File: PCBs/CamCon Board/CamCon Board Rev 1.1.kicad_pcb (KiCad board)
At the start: 2 copper layers, 25 x 25 mm, 28 parts, among them J1 SFW15R-1STE1LF

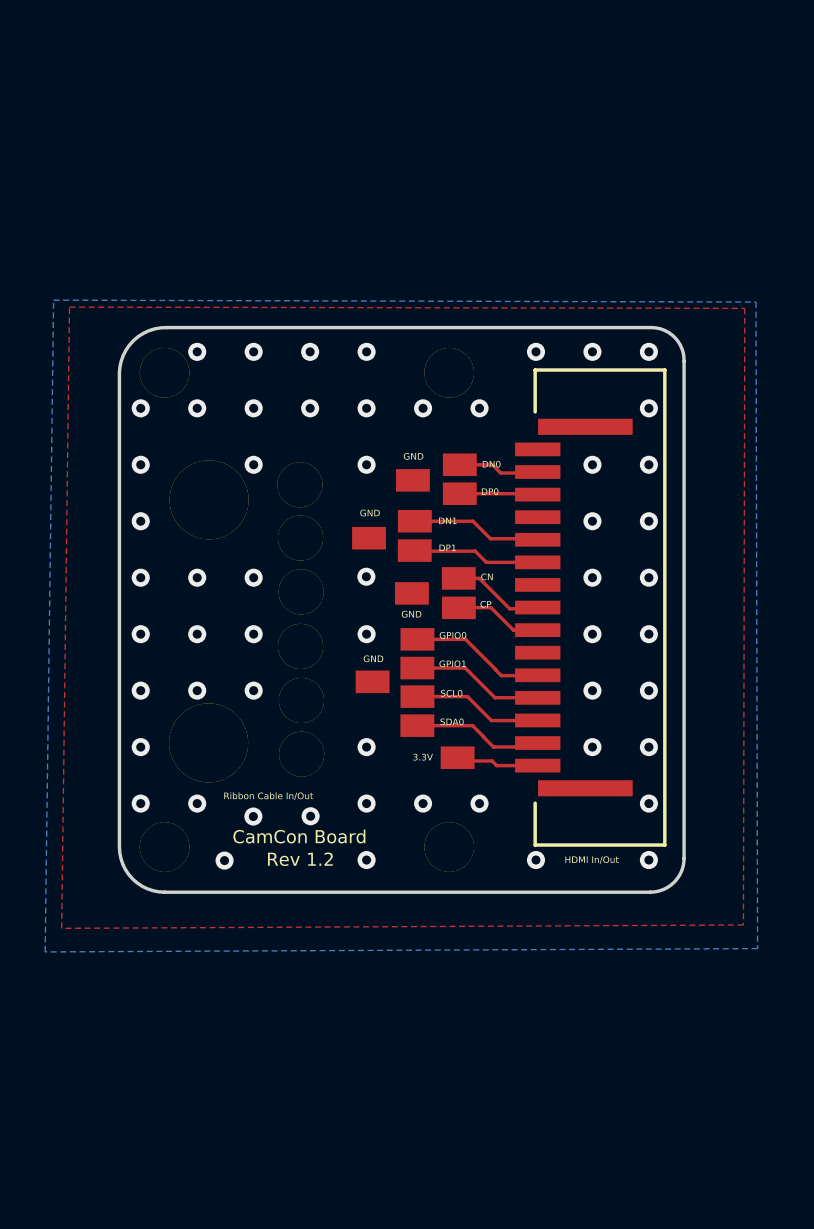
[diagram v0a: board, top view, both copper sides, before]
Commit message: More Gerbers
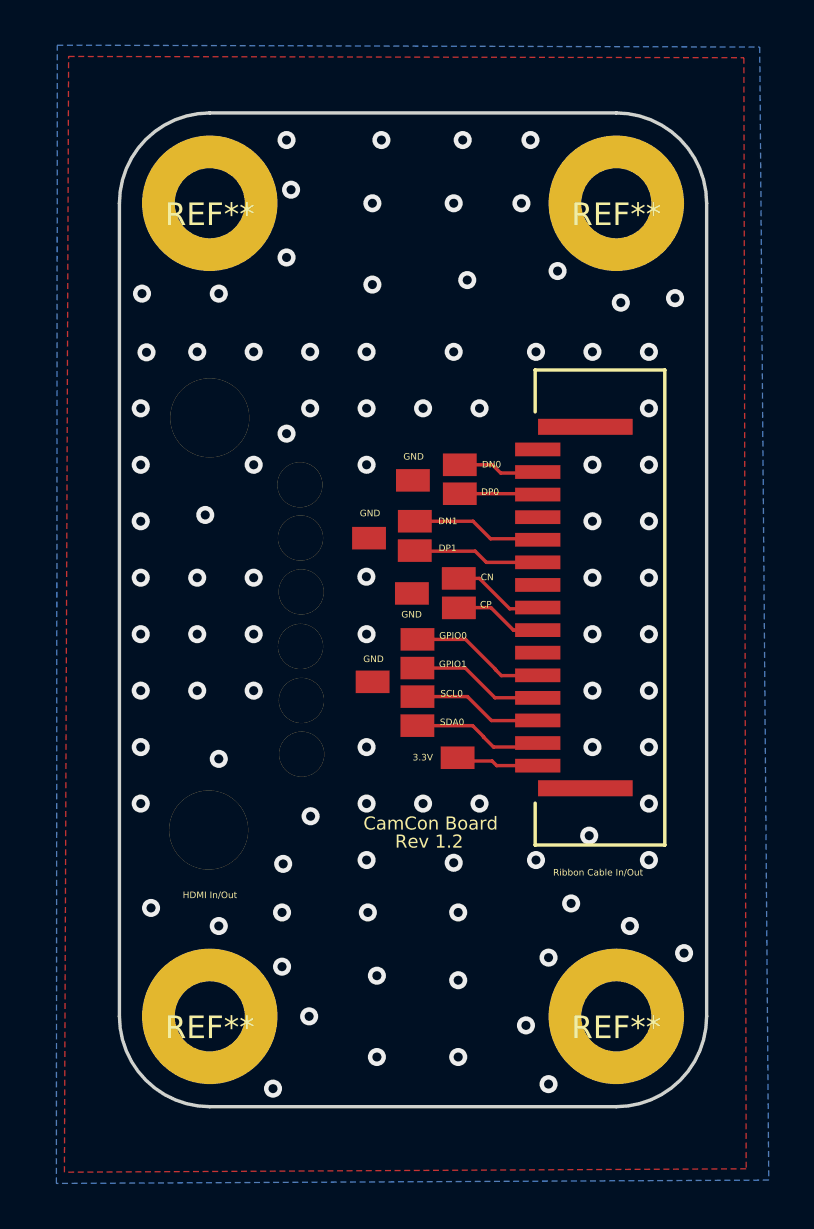
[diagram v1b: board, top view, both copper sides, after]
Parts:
- removed @HOLE0, @HOLE1, @HOLE2, @HOLE3: , 
- added REF**: M3STANDOFF, EER:M3STANDOFF, F.Cu at (140.0, 123.0)
- added REF**: M3STANDOFF, EER:M3STANDOFF, F.Cu at (158.0, 123.0)
- added REF**: M3STANDOFF, EER:M3STANDOFF, F.Cu at (158.0, 87.0)
- added REF**: M3STANDOFF, EER:M3STANDOFF, F.Cu at (140.0, 87.0)
- added U$12: EERLOGO, EER:EERLOGO, B.Cu at (145.8, 114.2)
- moved @HOLE11 3.86 mm to (140.0, 114.8)
- moved @HOLE10 3.63 mm to (140.0, 96.5)
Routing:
- net GND: vias 56 -> 93
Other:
- board size 25 x 25 mm -> 26 x 44 mm

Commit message: 3D Modeling
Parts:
- J1: footprint CamCon Board Rev 1.1:CON15_1X15_DRB_SFW -> EER:CON15_1X15_DRB_SFW
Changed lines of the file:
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@@
     (add_net "Net-(J1-Pad9)")
   )
-  (module EER:M3STANDOFF (layer Top)
-    (at 140 123)
-    (fp_text reference REF** (at 0 0.5) (layer F.SilkS)
-      (effects (font (size 1 1) (thickness 0.15)))
-    )
-    (fp_text value M3STANDOFF (at 0 -0.5) (layer F.Fab)
-      (effects (font (size 1 1) (thickness 0.15)))
-    )
-    (pad 1 thru_hole circle (at 0 0) (size 6 6) (drill 3.1) (layers *.Cu *.Mask))
-  )
-  (module EER:M3STANDOFF (layer Top)
-    (at 158 123)
-    (fp_text reference REF** (at 0 0.5) (layer F.SilkS)
-      (effects (font (size 1 1) (thickness 0.15)))
-    )
-    (fp_text value M3STANDOFF (at 0 -0.5) (layer F.Fab)
-      (effects (font (size 1 1) (thickness 0.15)))
-    )
-    (pad 1 thru_hole circle (at 0 0) (size 6 6) (drill 3.1) (layers *.Cu *.Mask))
-  )
-  (module EER:M3STANDOFF (layer Top)
-    (at 158 87)
-    (fp_text reference REF** (at 0 0.5) (layer F.SilkS)
-      (effects (font (size 1 1) (thickness 0.15)))
-    )
-    (fp_text value M3STANDOFF (at 0 -0.5) (layer F.Fab)
-      (effects (font (size 1 1) (thickness 0.15)))
-    )
-    (pad 1 thru_hole circle (at 0 0) (size 6 6) (drill 3.1) (layers *.Cu *.Mask))
-  )
-  (module "CamCon Board Rev 1.1:CON15_1X15_DRB_SFW" (layer Top)
+  (module EER:CON15_1X15_DRB_SFW (layer Top)
     (at 151.765669 104.898905 270)
     (fp_text reference J1 (at 0 0 270) (layer F.SilkS) hide
@@
     (pad 17 smd rect (at 8.001 -4.8641 270) (size 0.7112 4.191) (layers Top F.Paste F.Mask)
       (net 1 GND) (solder_mask_margin 0.1016))
-    (model "${KIPRJMOD}/3D Components/ssfw15r_2_4st_lf.stp"
-      (offset (xyz 0 8.5 0))
+    (model "../EERLibraries/3D Models/ssfw15r_1_3st_lf.STEP"
+      (offset (xyz -17.3 8.5 2.65))
       (scale (xyz 1 1 1))
-      (rotate (xyz -90 0 180))
+      (rotate (xyz 90 0 0))
     )
   )
+  (module EER:M3STANDOFF (layer Top)
+    (at 140 123)
+    (fp_text reference REF** (at 0 0.5) (layer F.SilkS)
+      (effects (font (size 1 1) (thickness 0.15)))
+    )
+    (fp_text value M3STANDOFF (at 0 -0.5) (layer F.Fab)
+      (effects (font (size 1 1) (thickness 0.15)))
+    )
+    (pad 1 thru_hole circle (at 0 0) (size 6 6) (drill 3.1) (layers *.Cu *.Mask))
+  )
+  (module EER:M3STANDOFF (layer Top)
+    (at 158 123)
+    (fp_text reference REF** (at 0 0.5) (layer F.SilkS)
+      (effects (font (size 1 1) (thickness 0.15)))
+    )
+    (fp_text value M3STANDOFF (at 0 -0.5) (layer F.Fab)
+      (effects (font (size 1 1) (thickness 0.15)))
+    )
+    (pad 1 thru_hole circle (at 0 0) (size 6 6) (drill 3.1) (layers *.Cu *.Mask))
+  )
+  (module EER:M3STANDOFF (layer Top)
+    (at 158 87)
+    (fp_text reference REF** (at 0 0.5) (layer F.SilkS)
+      (effects (font (size 1 1) (thickness 0.15)))
+    )
+    (fp_text value M3STANDOFF (at 0 -0.5) (layer F.Fab)
+      (effects (font (size 1 1) (thickness 0.15)))
+    )
+    (pad 1 thru_hole circle (at 0 0) (size 6 6) (drill 3.1) (layers *.Cu *.Mask))
+  )
   (module "" (layer Top)
